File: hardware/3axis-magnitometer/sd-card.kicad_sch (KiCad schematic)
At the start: 4 parts, among them J2 Micro_SD_Card

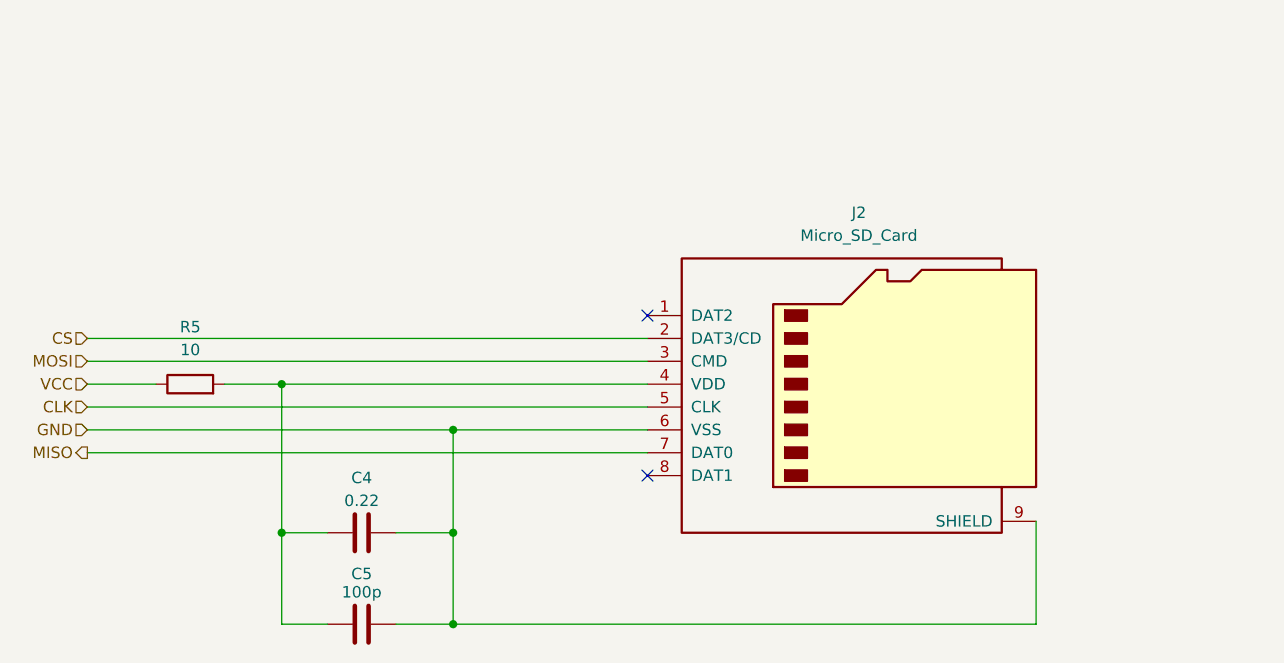
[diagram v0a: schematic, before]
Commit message: Add files via upload
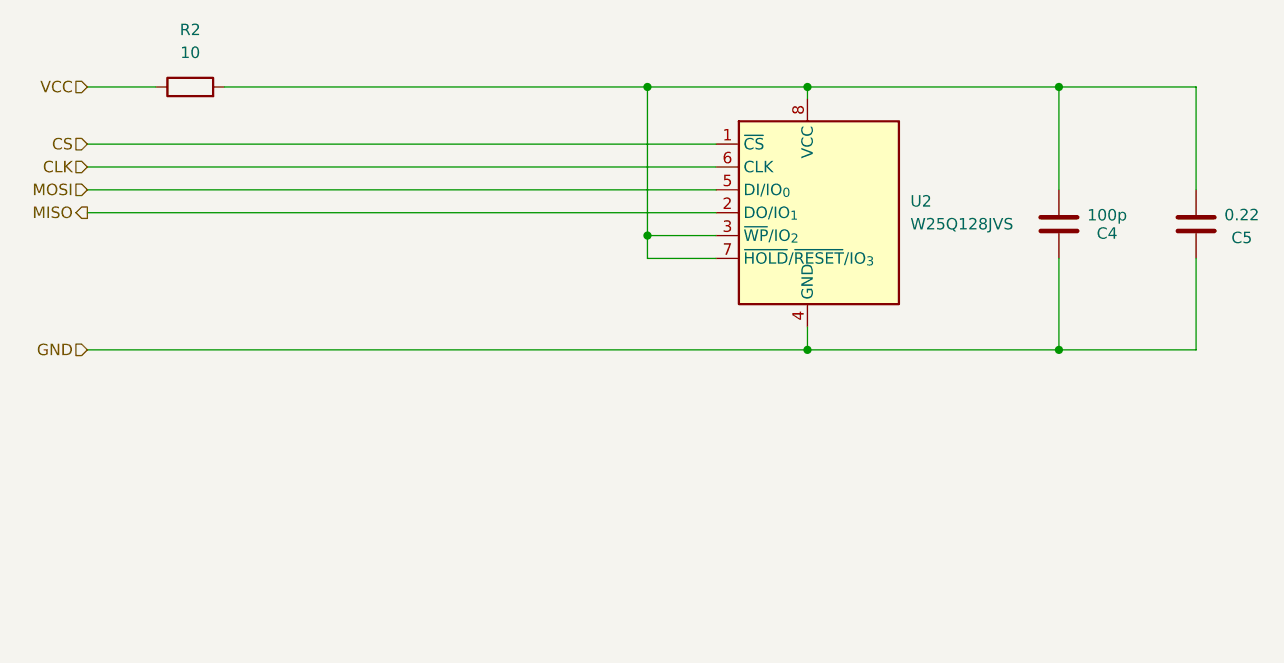
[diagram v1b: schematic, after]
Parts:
- removed J2: Micro_SD_Card, Connector_Card:microSD_HC_Molex_47219-2001, symbol Connector:Micro_SD_Card
- added U2: W25Q128JVS, Package_SO:SOIC-8_5.3x5.3mm_P1.27mm, symbol Memory_Flash:W25Q128JVS
- renumbered C5 to C4, C4 to C5, R5 to R2
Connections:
- net CLK: now also U2.6 (CLK)
- net CS: now also U2.1 (~{CS})
- net GND: now also U2.4 (GND)
- net MISO: now also U2.2 (DO/IO_{1})
- net MOSI: now also U2.5 (DI/IO_{0})
- net at C4.2, C5.2, R2.2: now also U2.3 (~{WP}/IO_{2}), U2.7 (~{HOLD}/~{RESET}/IO_{3}), U2.8 (VCC)
- no-connect marks 2 -> 0
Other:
- moved on the sheet: C4, C5, R2
